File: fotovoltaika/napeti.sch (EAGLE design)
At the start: 6 parts

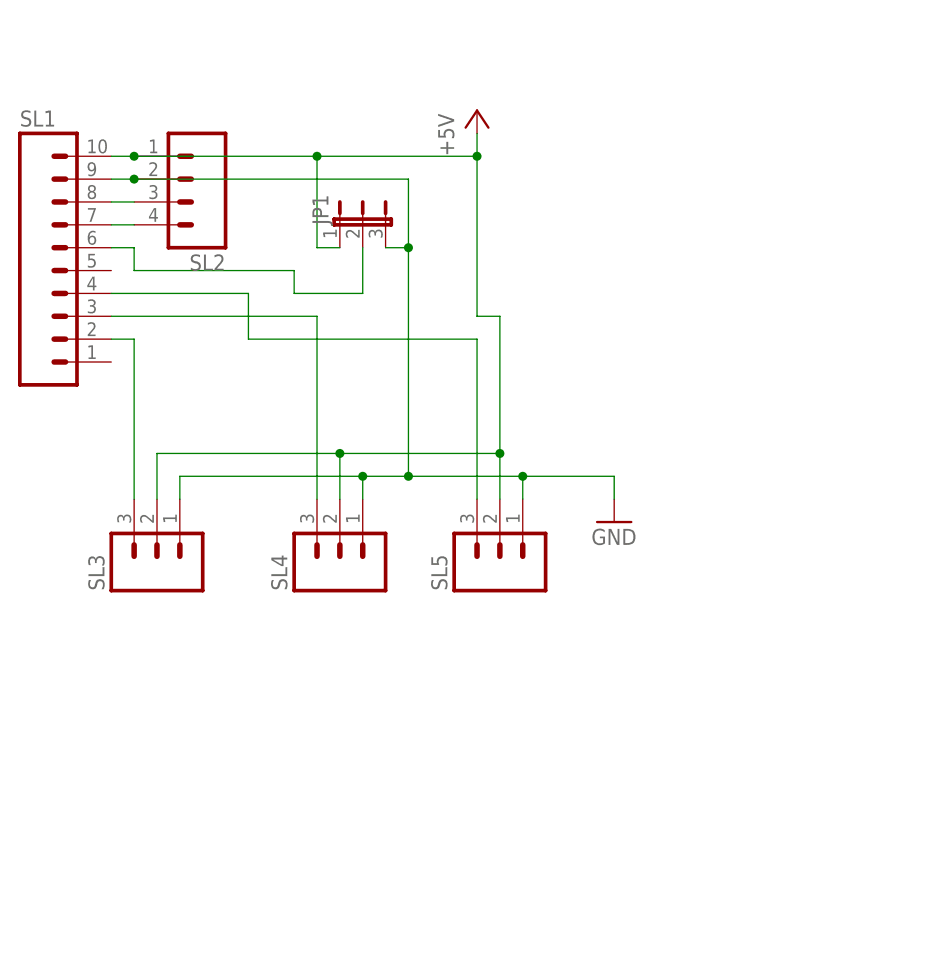
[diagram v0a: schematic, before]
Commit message: upravy desek
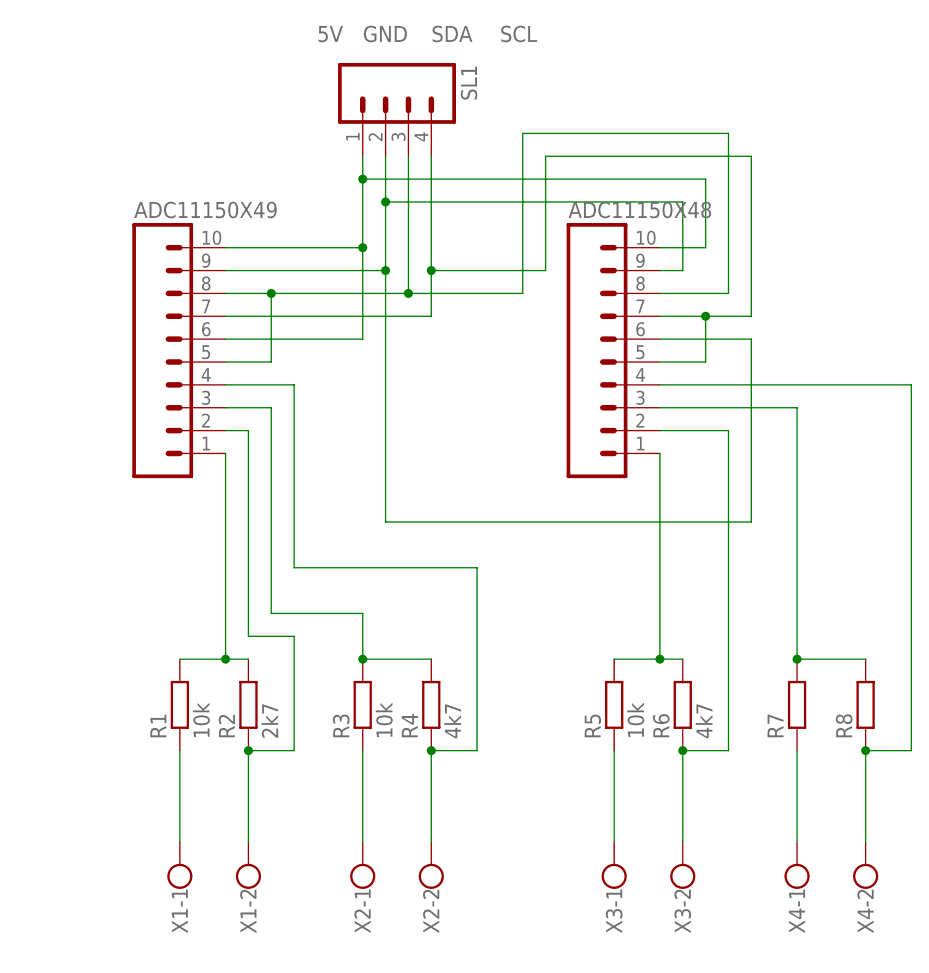
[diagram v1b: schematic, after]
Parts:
- removed JP1: (no value), jumper:JP2E
- removed SL2: (no value), con-amp-quick:M04
- removed SL3, SL4, SL5: (no value), con-amp-quick:M03
- added ADC11150X48, ADC11150X49: (no value), con-amp-quick:M10
- added R1, R3, R5: 10k, rcl:R-EU_0204/7
- added R2: 2k7, rcl:R-EU_0204/7
- added R4, R6: 4k7, rcl:R-EU_0204/7
- added R7, R8: (no value), rcl:R-EU_0204/7
- added X1, X2, X3, X4: (no value), con-wago-500:W237-102
- SL1: device con-amp-quick:M10 -> con-amp-quick:M04
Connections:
- removed net +5V: JP1.1, SL1.10, SL2.1, SL3.2, SL4.2, SL5.2
- removed net N$11: SL1.7, SL2.4
- new net 5V: ADC11150X48.10, ADC11150X49.10, ADC11150X49.6, SL1.1
- new net N$1: ADC11150X48.1, R5.2, R6.2
- new net N$10: ADC11150X49.2, R2.1, X1-2.KL
- new net N$13: ADC11150X49.3, R3.2, R4.2
- new net N$3: ADC11150X48.2, R6.1, X3-2.KL
- new net N$4: ADC11150X48.3, R7.2, R8.2
- new net N$8: R7.1, X4-1.KL
- new net N$9: ADC11150X49.1, R1.2, R2.2
- new net SCL: ADC11150X48.5, ADC11150X48.7, ADC11150X49.7, SL1.4
- new net SDA: ADC11150X48.8, ADC11150X49.5, ADC11150X49.8, SL1.3
- net GND: now also ADC11150X48.6, ADC11150X48.9, ADC11150X49.9, SL1.2; no longer JP1.3, SL1.9, SL2.2, SL3.1, SL4.1, SL5.1
- net N$14: now also ADC11150X49.4, R4.1, X2-2.KL; no longer JP1.2, SL1.6
- net N$2: now also R1.1, X1-1.KL; no longer SL1.8, SL2.3
- net N$5: now also R3.1, X2-1.KL; no longer SL1.2, SL3.3
- net N$6: now also ADC11150X48.4, R8.1, X4-2.KL; no longer SL1.3, SL4.3
- net N$7: now also R5.1, X3-1.KL; no longer SL1.4, SL5.3
